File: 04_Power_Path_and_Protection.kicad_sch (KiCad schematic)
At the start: 12 parts, among them J3 PACK+ M4, J4 PACK- M4

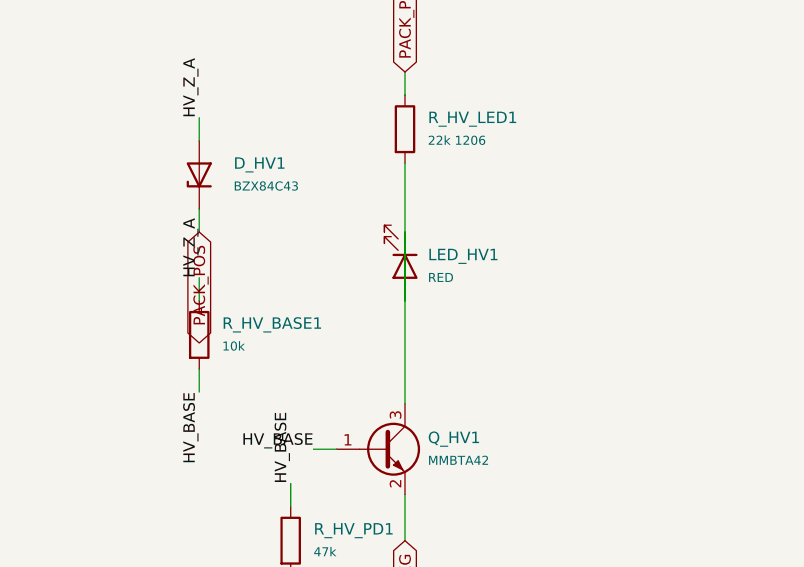
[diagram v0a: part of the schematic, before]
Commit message: just tested
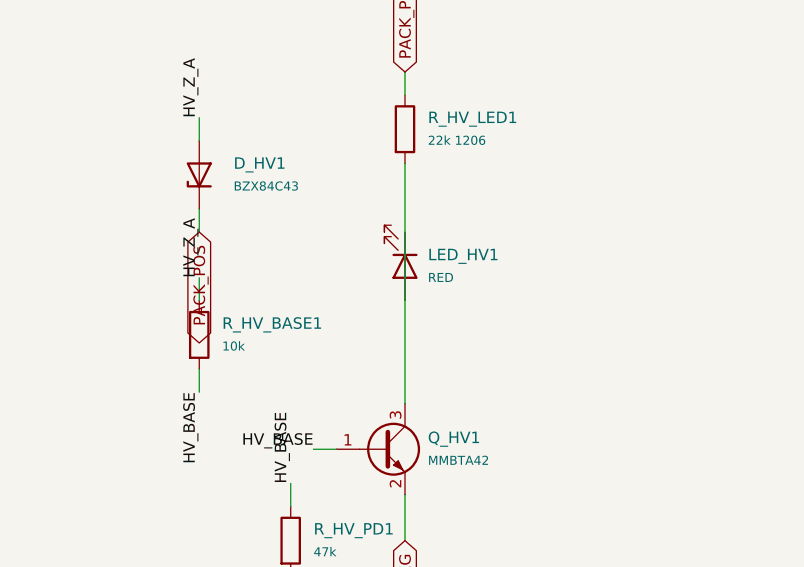
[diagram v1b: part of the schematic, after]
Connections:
- net at Q_HV1.3 (C), R_HV_LED1.2: no longer LED_HV1.1 (K), LED_HV1.2 (A)
